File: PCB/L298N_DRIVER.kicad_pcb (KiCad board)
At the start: 2 copper layers, 64.8 x 43.5 mm, 23 parts, among them J1 PWM-A, J2 MOT1, J3 +5V, J4 +BATT, J5 SERIAL, J6 I2C, J7 MOT02, J8 PWM-B, U1 L298N, U2 adino2

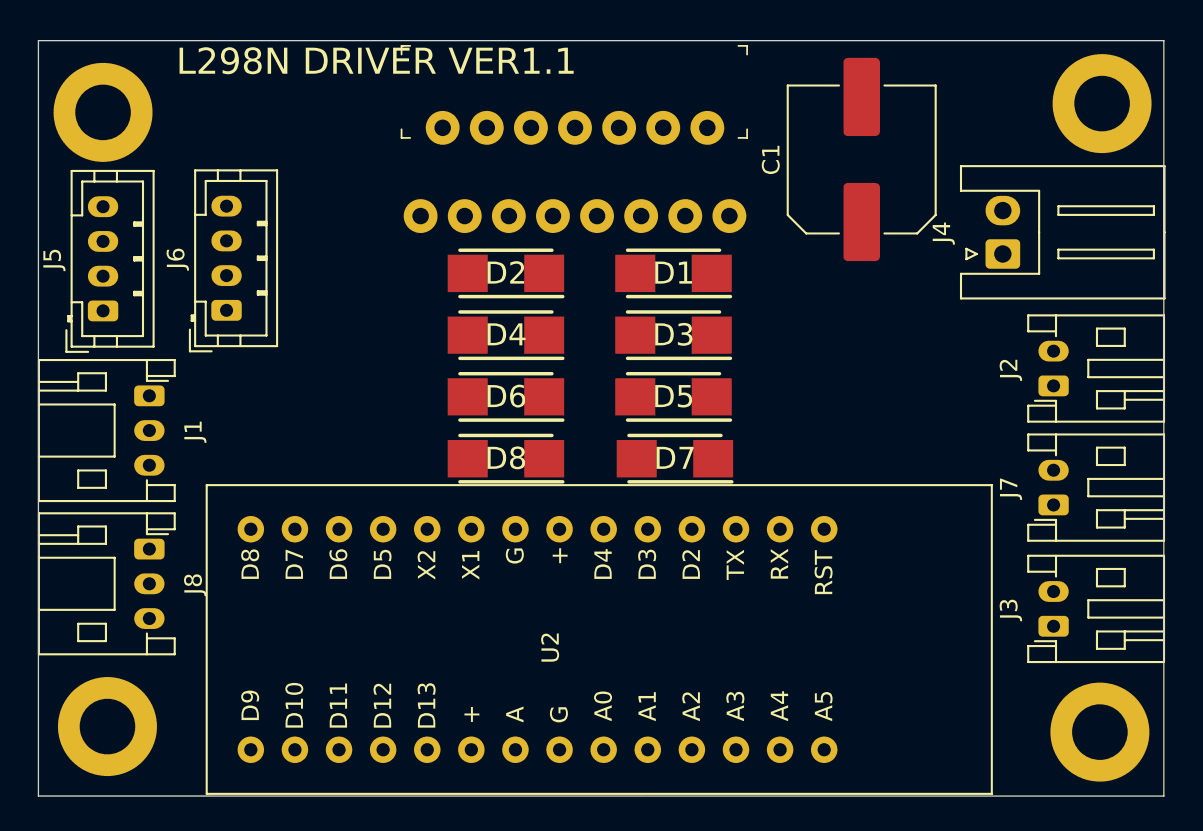
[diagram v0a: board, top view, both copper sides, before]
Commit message: bug fix
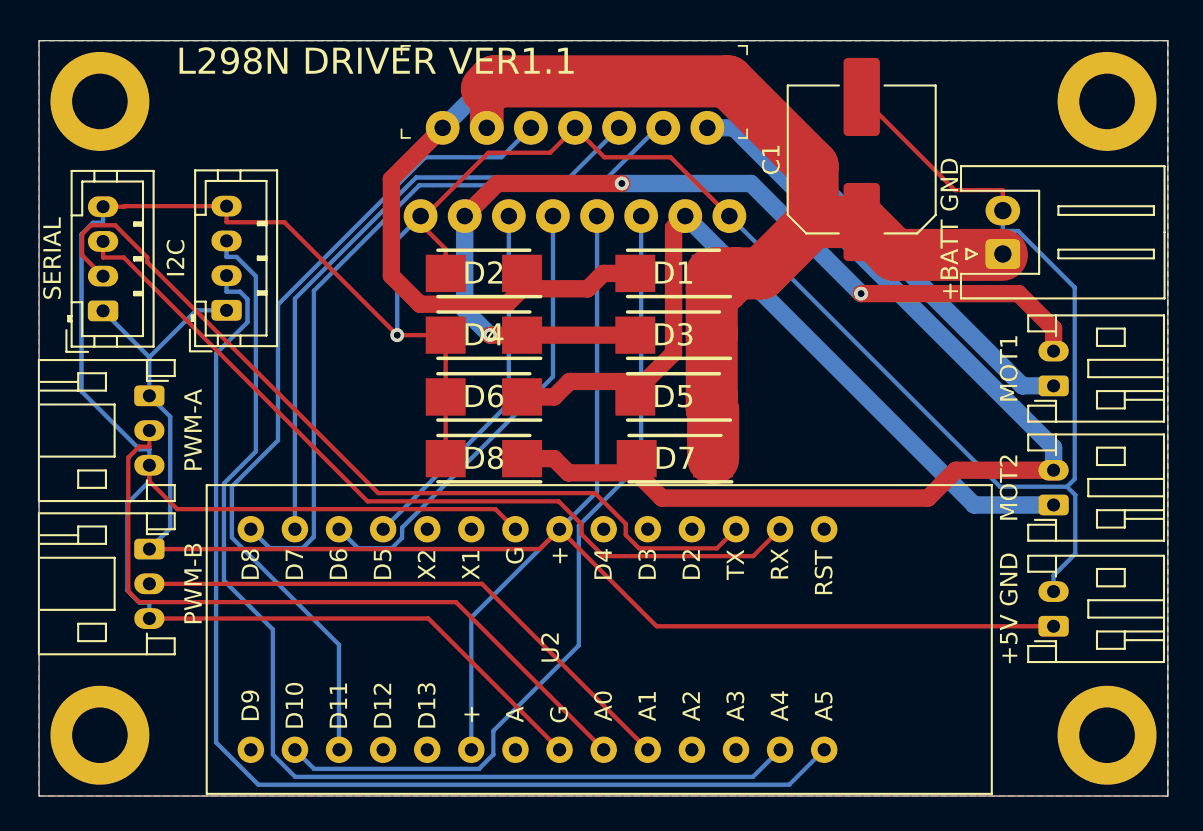
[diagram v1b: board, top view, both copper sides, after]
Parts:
- +5V GND: renamed from J3
- +BATT GND: renamed from J4
- moved D2 1.27 mm to (144.6, 57.4)
- moved D4 1.27 mm to (144.6, 61.0)
- moved D6 1.27 mm to (144.6, 64.5)
- moved D8 1.27 mm to (144.6, 68.1)
- moved H3 0.66 mm to (122.5, 47.5)
- moved H4 0.46 mm to (123.3, 83.2)
- moved H2 0.31 mm to (180.5, 47.5)
- moved H1 0.20 mm to (180.0, 84.0)
- renumbered J6 to I2C, J2 to MOT1, J7 to MOT2, J1 to PWM-A, J8 to PWM-B, J5 to SERIAL
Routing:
- net GND: track 0.00 -> 204.0 mm, vias 0 -> 1
- net +5V: track 0.00 -> 110.0 mm
- net /OUT1: track 0.00 -> 68.8 mm
- net /SCL: track 0.00 -> 65.4 mm
- net /SDA: track 0.00 -> 62.9 mm
- net /OUT4: track 0.00 -> 61.9 mm
- net +BATT: track 0.00 -> 56.9 mm
- net /OUT2: track 0.00 -> 55.3 mm, vias 0 -> 3
- net /TX: track 0.00 -> 49.5 mm
- net /EN_A: track 0.00 -> 48.1 mm
- net /RX: track 0.00 -> 48.0 mm
- net /OUT3: track 0.00 -> 46.9 mm
- net /EN_B: track 0.00 -> 46.8 mm
- net /IN4: track 0.00 -> 42.5 mm
- net /PWM_A: track 0.00 -> 41.3 mm
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- added copper zone on B.Cu, net GND
- added copper zone on F.Cu, net GND
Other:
- board size 64.8 x 43.5 mm -> 65 x 43.5 mm
